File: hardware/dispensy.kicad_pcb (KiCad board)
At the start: 2 copper layers, 125 x 90 mm, 96 parts, among them SW1 BOOTSEL, SW2 RESET, SW3 UP, SW4 MENU, SW5 DOWN, U1 DBT50G-7_62-4P, U10 RP2040, U11 SS54_C22452, U12 SS54_C22452, U13 CAN_IO, U14 TJA1042T_3_1J, U15 USB-C, U16 LM2576S-5_0_TR, U17 100uH, U18 XY300V-A-5_0-2P, U2 USB-A, U3 LM2576S-5_0_TR, U4 100uH, U5 AMS1117-3_3_C347222, U6 SKCR-16S, U7 WS2812E-V5, U8 W25Q128JVSIQ, U9 74HC165D,653, X1 12MHz

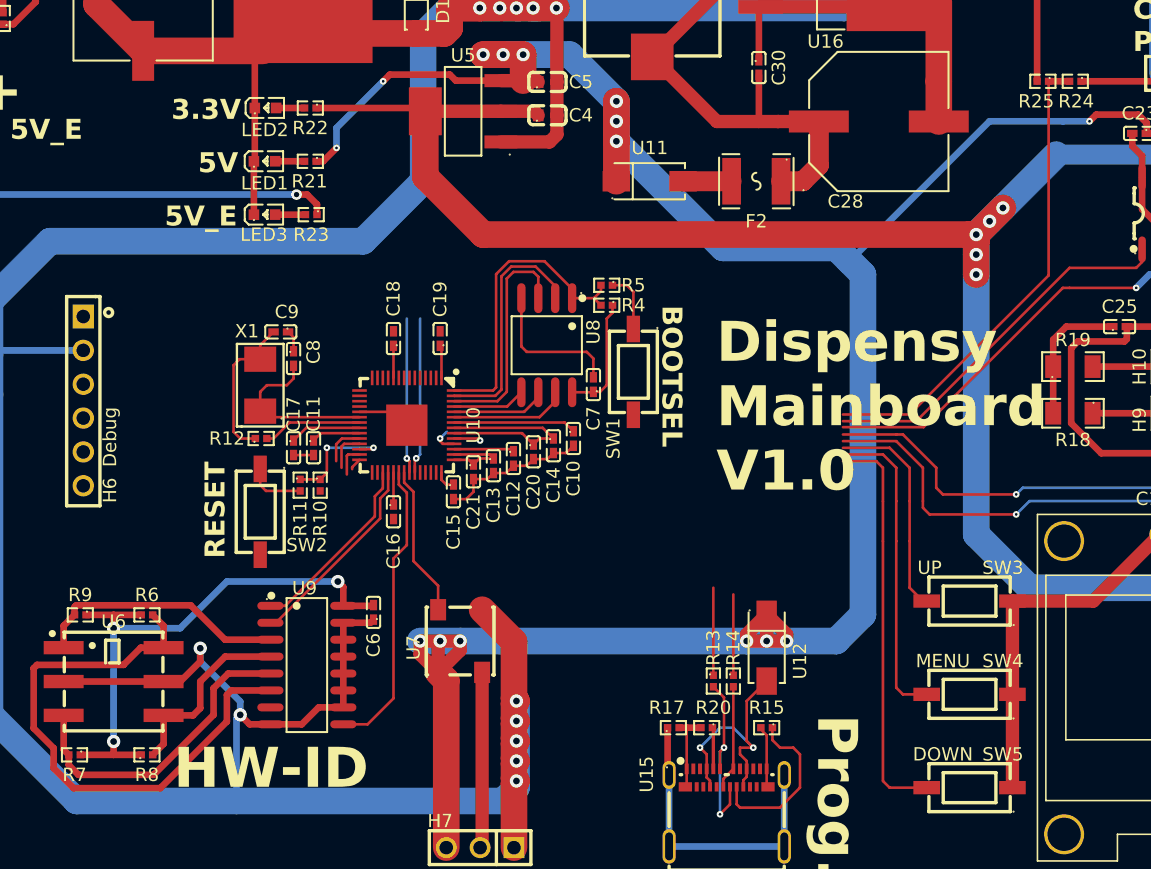
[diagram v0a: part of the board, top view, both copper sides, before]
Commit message: routing nearly finished
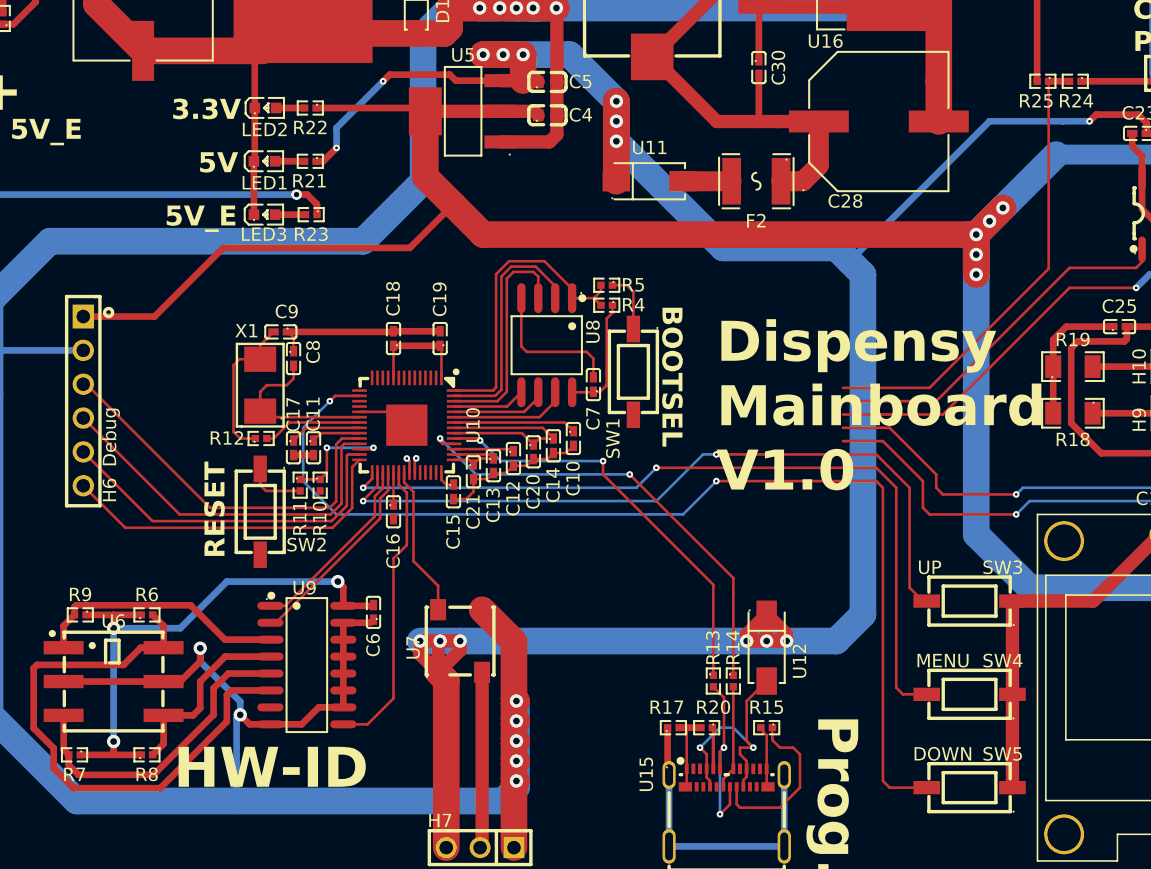
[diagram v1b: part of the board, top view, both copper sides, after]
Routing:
- net /PI/IO13: track 30.2 -> 80.5 mm, vias 0 -> 2
- net /PI/IO15: track 16.3 -> 55.3 mm, vias 0 -> 2
- net /PI/IO14: track 23.4 -> 60.2 mm, vias 0 -> 2
- net +3.3V: track 237.6 -> 272.3 mm
- net Net-(U10-USB_DM): track 8.11 -> 35.0 mm, vias 1 -> 2
- net /PI/Debug_Clock: track 3.19 -> 29.2 mm
- net /PI/Debug_Data: track 3.03 -> 28.4 mm
- net /PI/Debug_Rx: track 0.93 -> 25.9 mm
- net /PI/Debug_Tx: track 2.39 -> 27.1 mm
- net Net-(U10-USB_DP): track 8.58 -> 31.4 mm, vias 1 -> 2
- net GND: track 702.4 -> 713.9 mm
- net Net-(U10-GPIO24): track 40.0 -> 28.8 mm
- net Net-(U10-GPIO25): track 44.5 -> 33.4 mm
- net /PI/ADC0: track 35.9 -> 34.8 mm
- net /PI/I2C_SCL: track 37.7 -> 37.1 mm
